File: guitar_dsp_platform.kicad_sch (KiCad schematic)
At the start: 0 parts

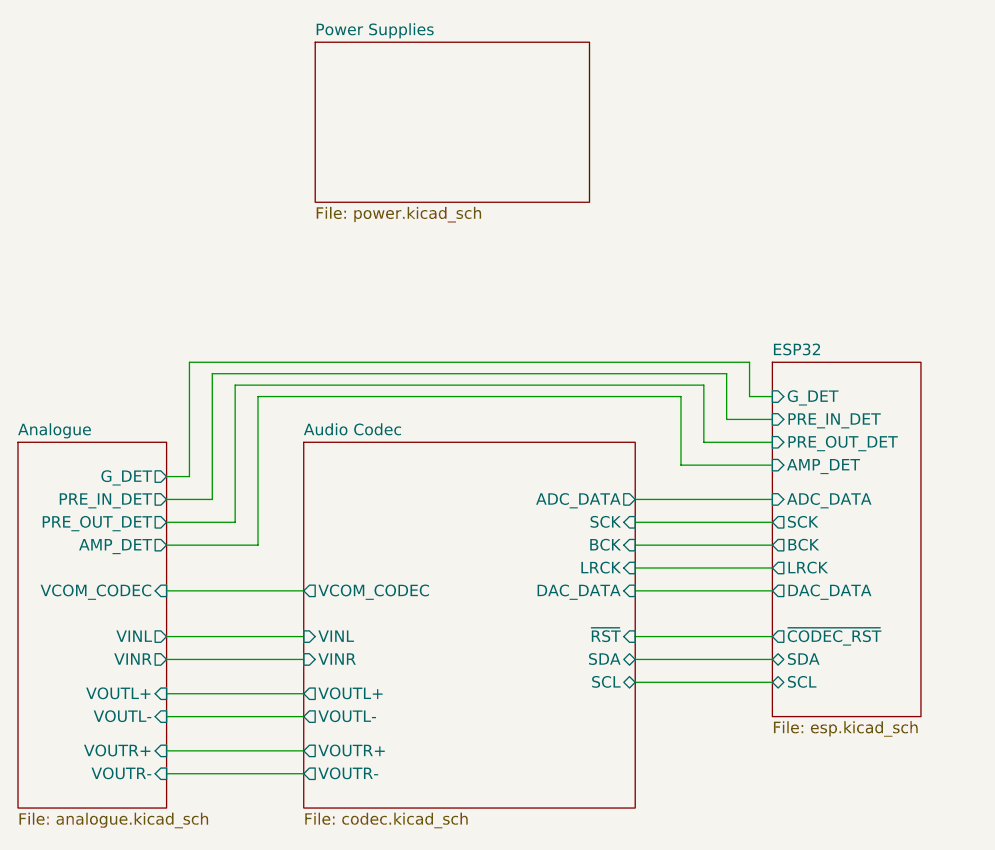
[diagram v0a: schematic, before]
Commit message: Working on schematic
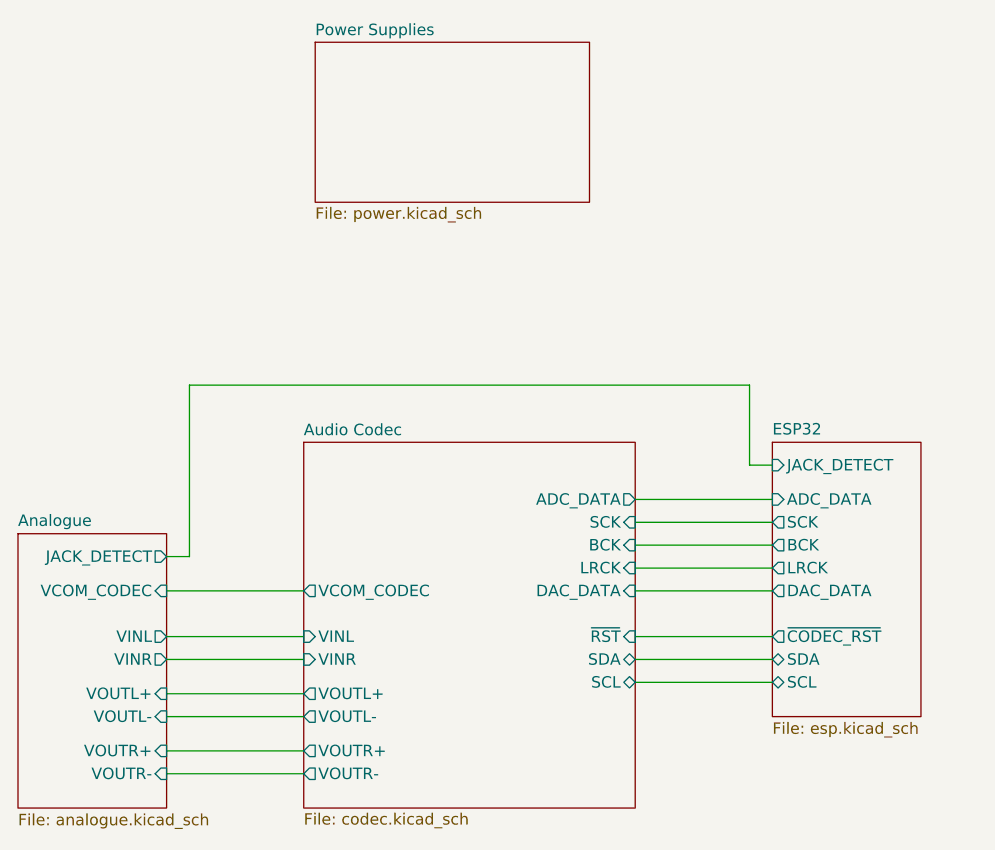
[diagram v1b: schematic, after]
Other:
- sheet Analogue ports: added JACK_DETECT; removed AMP_DET, G_DET, PRE_IN_DET, PRE_OUT_DET
- sheet ESP32 ports: added JACK_DETECT; removed AMP_DET, G_DET, PRE_IN_DET, PRE_OUT_DET
